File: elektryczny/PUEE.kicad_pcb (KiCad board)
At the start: 2 copper layers, 57 parts, among them J1 CAN, J2 VIN, J7 STM, SW1 Button2, SW2 Button1, U1 STM32F042F4Px, U10 WS2815, U11 WS2815, U13 SN65HVD230QDRG4Q1, U2 ESP-12E, U3 TPS54308, U4 WS2815, U5 WS2815, U6 WS2815, U7 WS2815, U8 WS2815, U9 WS2815, Y2 ABL-8MHZ-B2

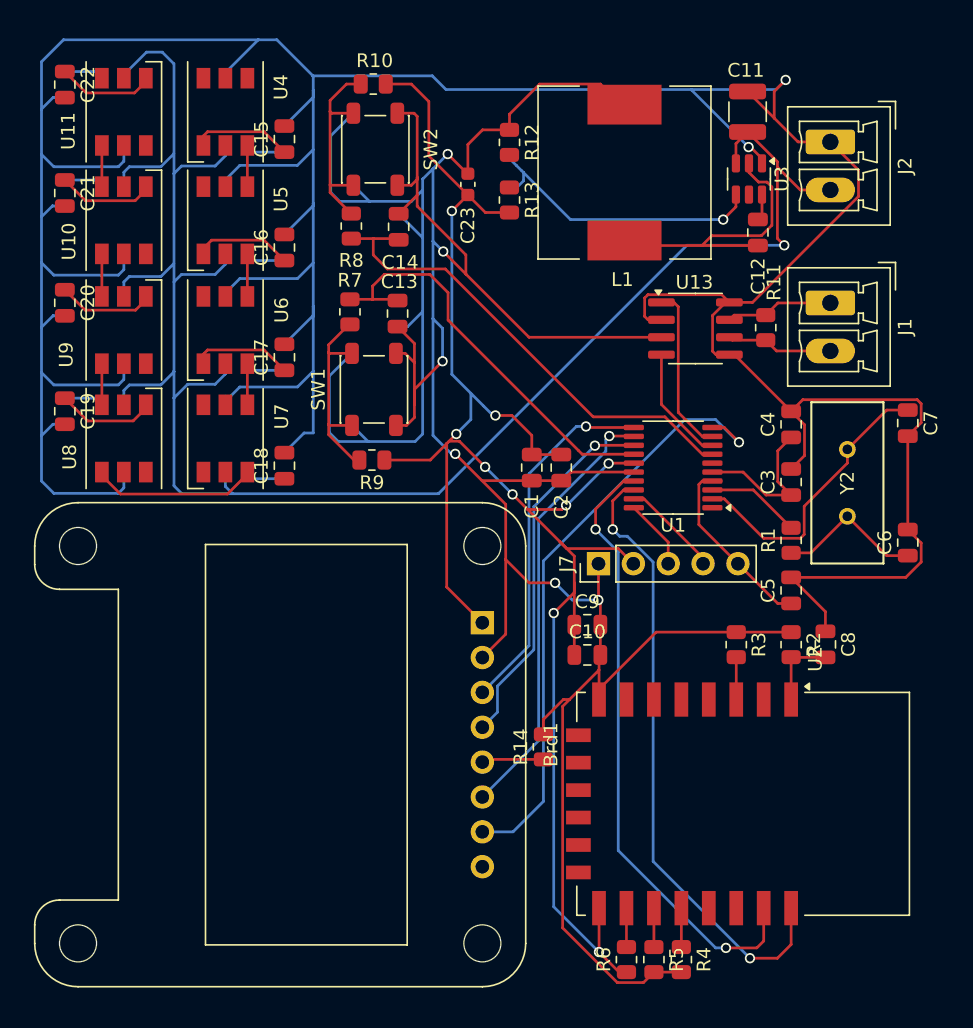
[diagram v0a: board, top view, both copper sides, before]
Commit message: finalizacja projektu v1.0
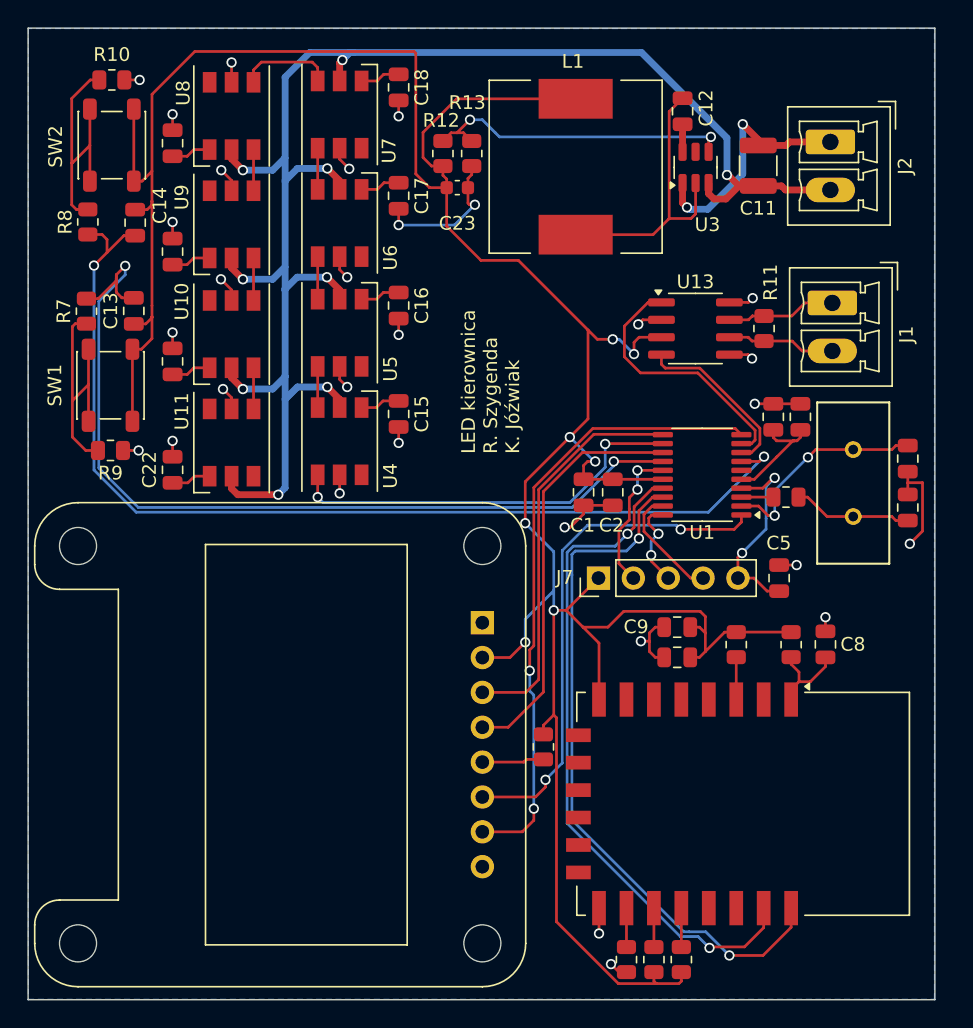
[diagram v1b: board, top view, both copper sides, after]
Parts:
- moved C22 29.1 mm to (123.9, 78.7), turned to 90 degrees
- moved C18 28.8 mm to (140.4, 50.8), turned to -90 degrees
- moved U4 25.4 mm to (136.1, 76.6), turned to -90 degrees
- moved U11 25.3 mm to (128.2, 76.7), turned to 90 degrees
- moved U7 25.0 mm to (136.1, 52.8), turned to -90 degrees
- moved U8 24.8 mm to (128.2, 52.9), turned to 90 degrees
- moved C15 21.7 mm to (140.4, 74.6), turned to -90 degrees
- moved C19 21.0 mm to (123.9, 54.9), turned to 90 degrees
- moved C13 19.2 mm to (121.1, 67.1)
- moved C14 19.2 mm to (121.2, 60.6)
- moved R8 19.2 mm to (117.8, 60.6)
- moved SW1 19.2 mm to (119.4, 72.5)
- moved SW2 19.2 mm to (119.5, 55.0)
- moved R7 19.2 mm to (117.7, 67.1)
- moved R9 19.1 mm to (119.4, 77.2)
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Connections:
- J1 pad 1: /CAN_L -> /CAN_H
- J1 pad 2: /CAN_H -> /CAN_L
- U1 pad 1: /GPIO_LED_RELAY1 -> /GPIO_OLED
- U1 pad 12: /GPIO_OLED -> /GPIO_LED_RELAY1
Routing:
- net -12V: track 424.5 -> 94.3 mm, vias 11 -> 34
- net /GPIO_Button1: track 35.4 -> 74.9 mm, vias 0 -> 2
- net /GPIO_Button2: track 30.6 -> 66.5 mm, vias 0 -> 2
- net VDD: track 250.0 -> 219.6 mm, vias 6 -> 7
- net /GPIO_LED_RELAY1: track 0.00 -> 29.7 mm, vias 0 -> 2
- net +12V: track 137.4 -> 119.6 mm, vias 1 -> 9
- net Net-(U6-NC): track 10.2 -> 2.90 mm
- net Net-(U4-NC): track 10.2 -> 2.90 mm
- net Net-(U8-NC): track 10.1 -> 2.90 mm
- net Net-(U5-NC): track 10.1 -> 2.90 mm
- net Net-(U11-NC): track 10.0 -> 2.90 mm
- net Net-(U10-NC): track 10.00 -> 2.90 mm
- net /USART2_RX: track 12.3 -> 19.2 mm
- net Net-(U1-PF0): track 21.1 -> 15.6 mm, vias 0 -> 2
- net /USART1_RX: track 45.7 -> 51.2 mm
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- added copper zone on B.Cu, net -12V
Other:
- board outline added: 66.1 x 70.8 mm
- board text added: "LED kierownica R. Szygenda K. Jóźwiak"
